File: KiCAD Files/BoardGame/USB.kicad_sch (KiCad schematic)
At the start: 12 parts, among them J201 USB_C_Receptacle_USB2.0, U201 USBLC6-2SC6, U202 CH340C

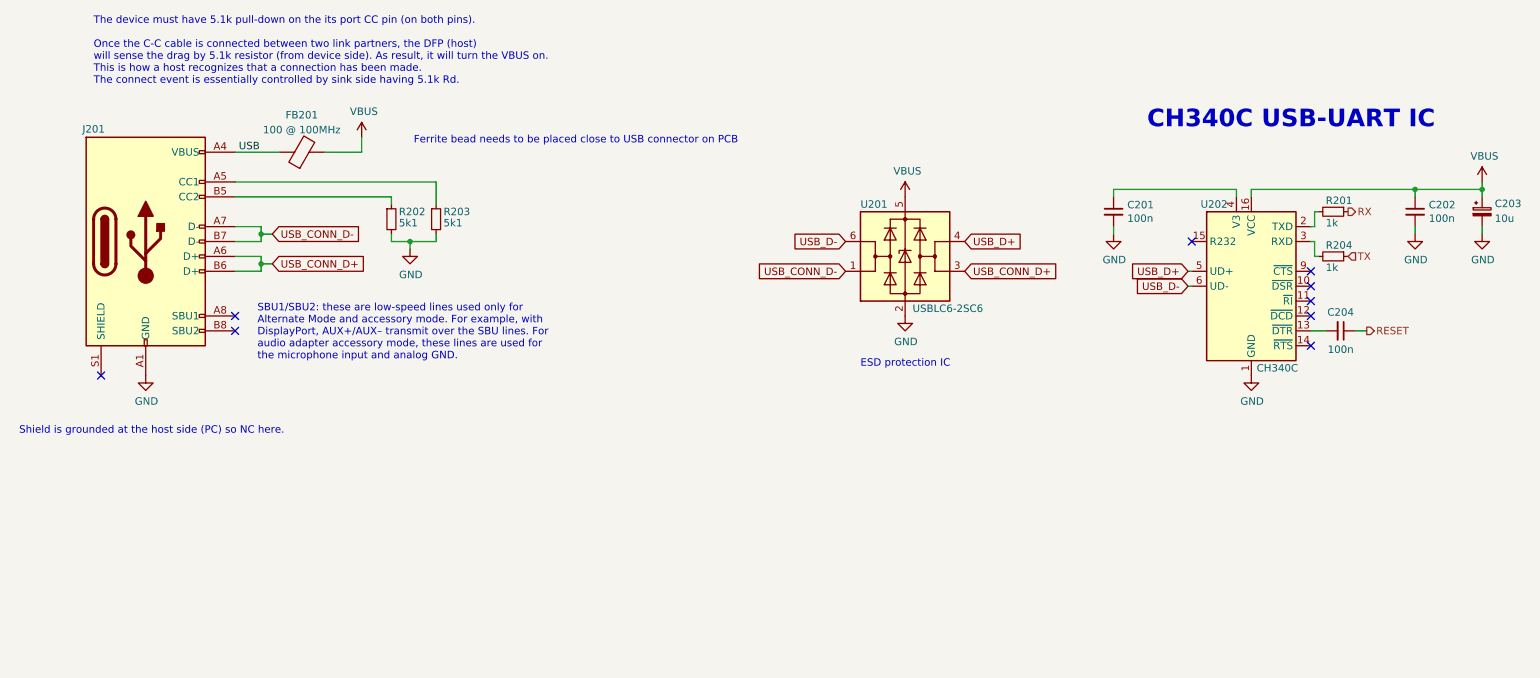
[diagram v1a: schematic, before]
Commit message: update
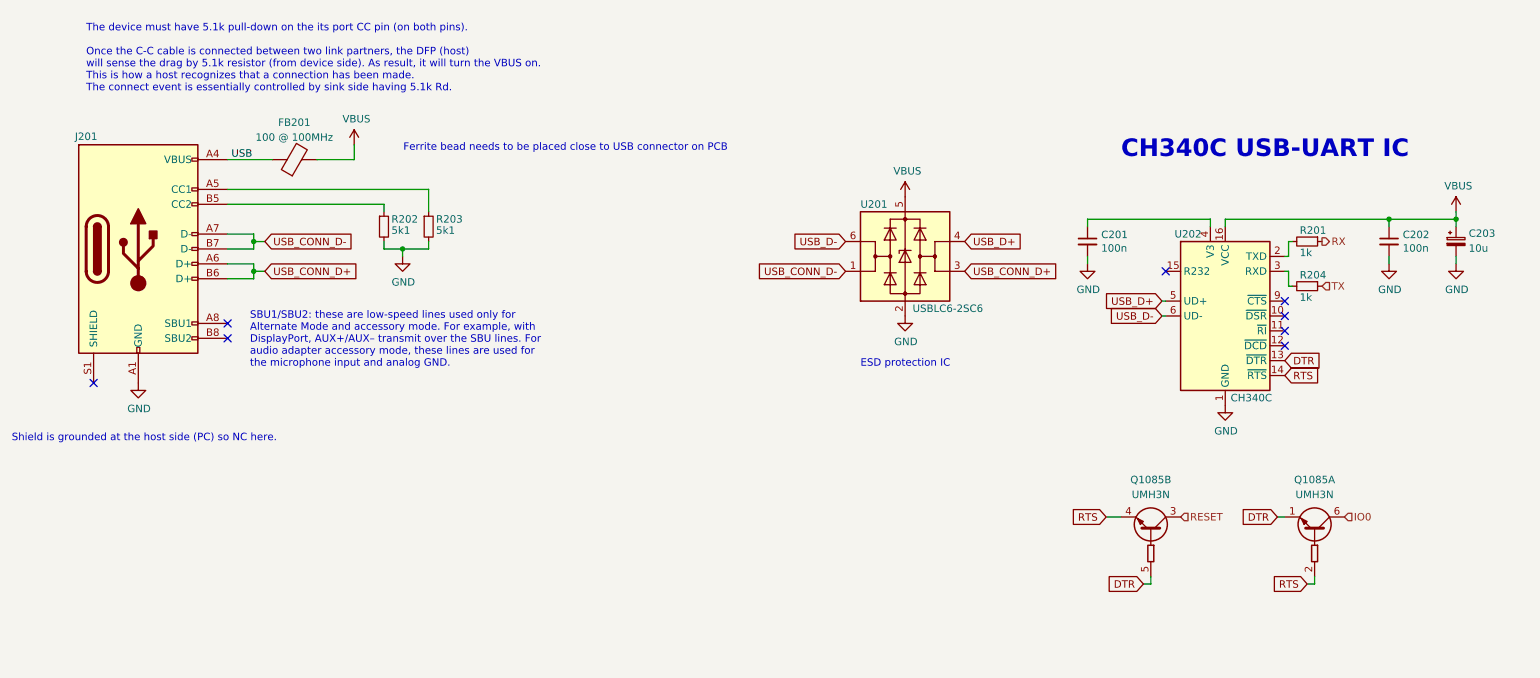
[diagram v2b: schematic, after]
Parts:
- removed C204: 100n, Capacitor_SMD:C_0603_1608Metric, symbol Device:C_Small
- added Q1085: UMH3N, Package_TO_SOT_SMD:SOT-363_SC-70-6, symbol Transistor_BJT:UMH3N
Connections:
- net RESET: now also Q1085.3 (C2)
- net DTR: now reaches U202.13 (~{DTR})
- net DTR: now also Q1085.1 (E1), Q1085.5 (B2)
- net RTS: now reaches U202.14 (~{RTS})
- net RTS: now also Q1085.2 (B1), Q1085.4 (E2)
- new net IO0: Q1085.6 (C1)
- no-connect marks 9 -> 8
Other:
- moved on the sheet: C201, C202, C203, FB201, J201, R201, R202, R203, R204, U202

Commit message: update
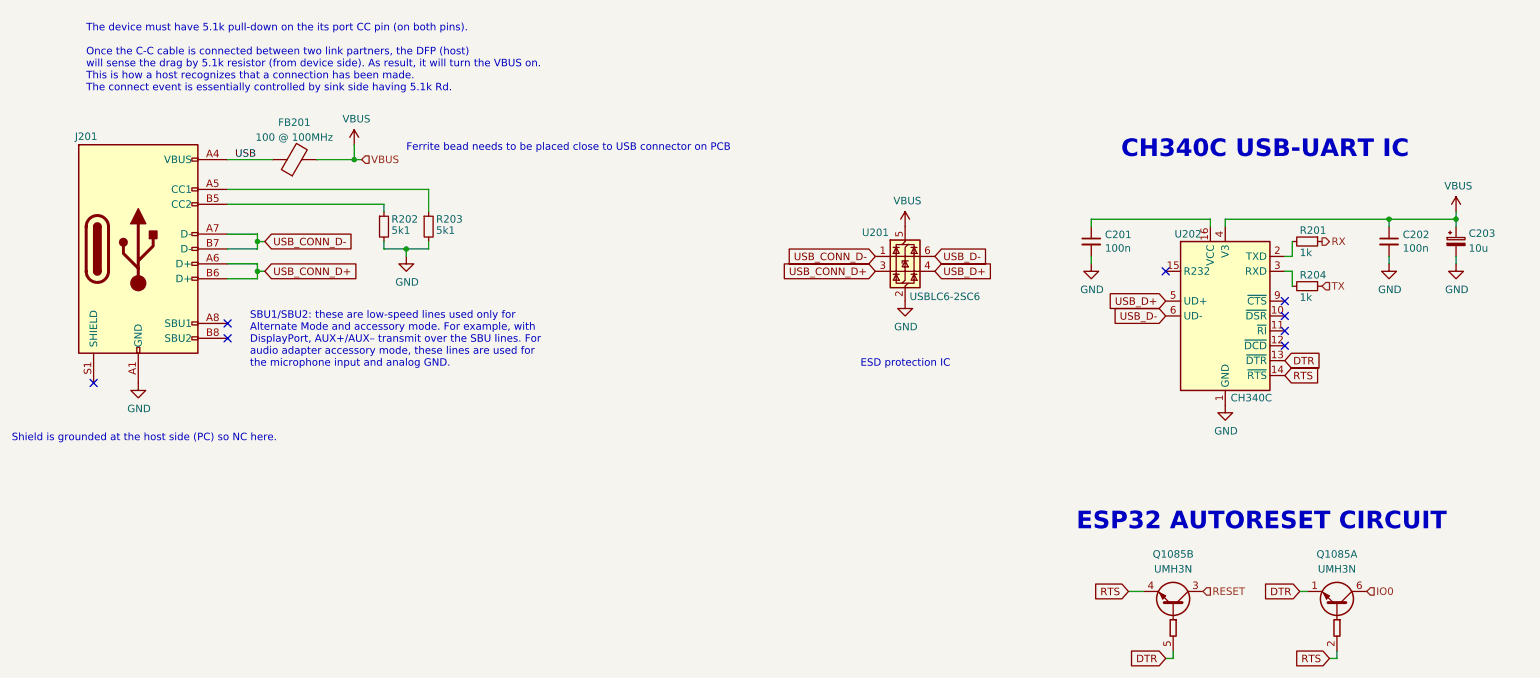
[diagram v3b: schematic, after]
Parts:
- J201: symbol Connector:USB_C_Receptacle_USB2.0 -> Connector:USB_C_Receptacle_USB2.0_16P
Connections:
- net VBUS: now also U202.4 (V3); no longer U202.16 (VCC)
- net at C201.1: now also U202.16 (VCC); no longer U202.4 (V3)
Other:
- note added: "ESP32 AUTORESET CIRCUIT"
- moved on the sheet: C201, Q1085A, Q1085B

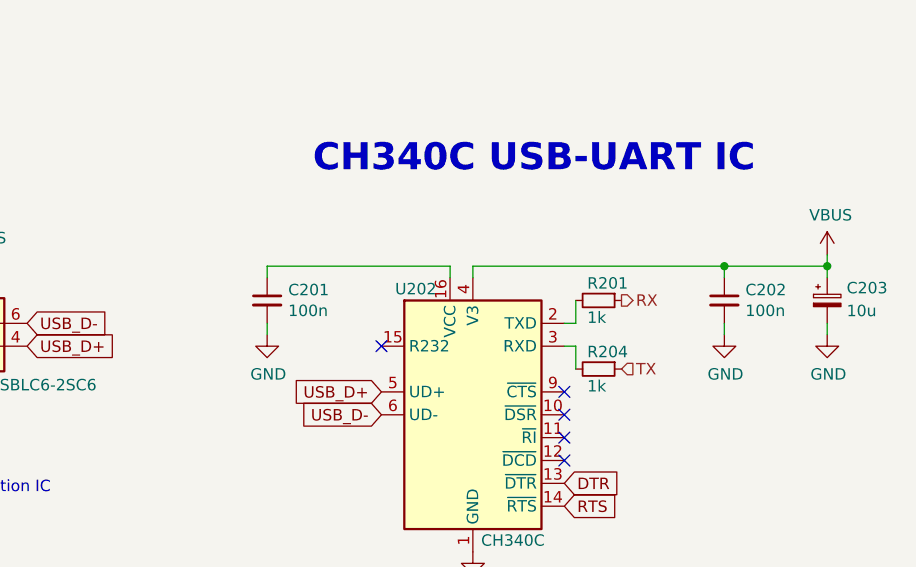
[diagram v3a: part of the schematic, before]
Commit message: update
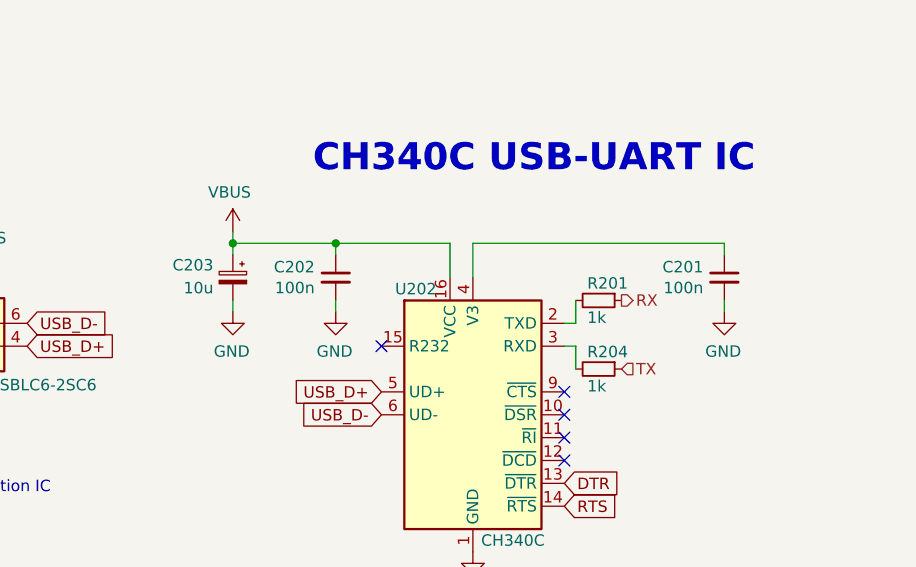
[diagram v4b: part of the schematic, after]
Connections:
- net VBUS: now also U202.16 (VCC); no longer U202.4 (V3)
- net at C201.1: now also U202.4 (V3); no longer U202.16 (VCC)
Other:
- moved on the sheet: C201, C202, C203
